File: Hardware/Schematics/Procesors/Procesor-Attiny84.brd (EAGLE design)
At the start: 27.9 x 27.9 mm, 6 parts

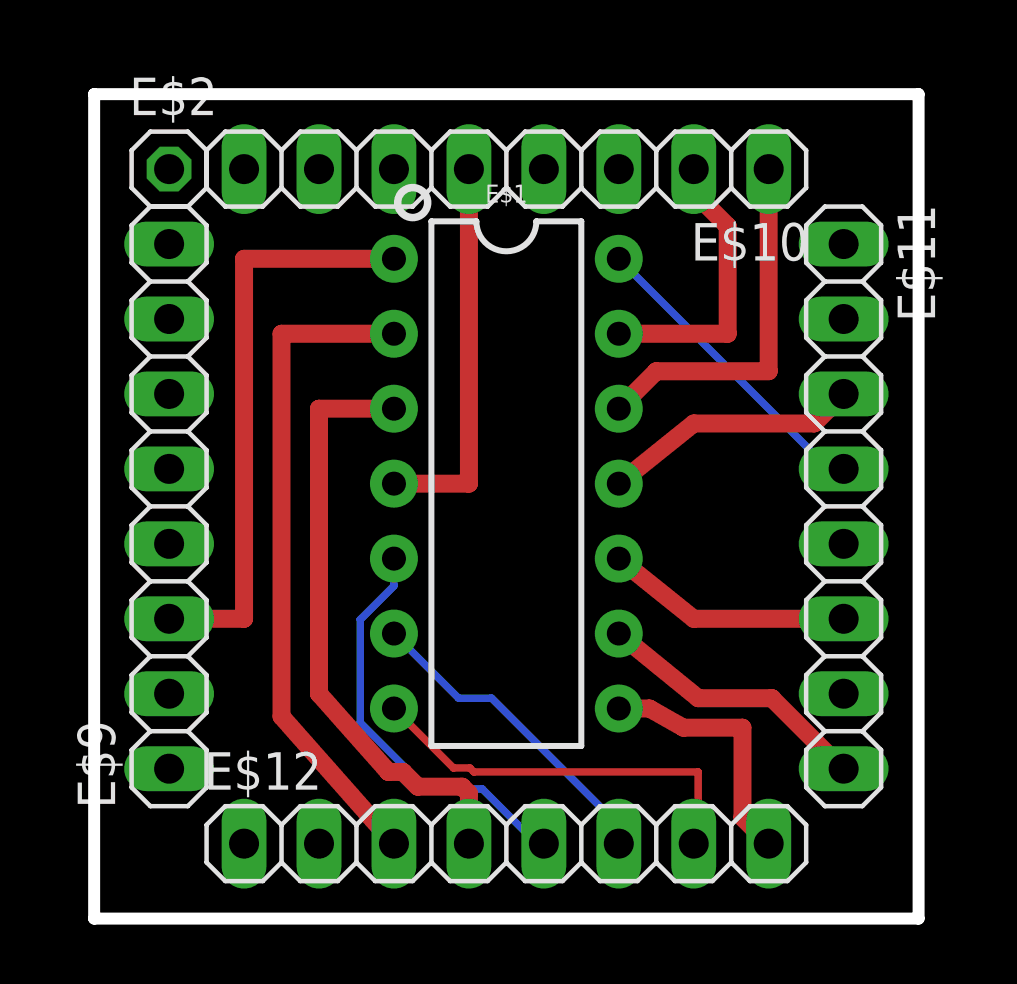
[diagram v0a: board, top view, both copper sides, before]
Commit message: commit
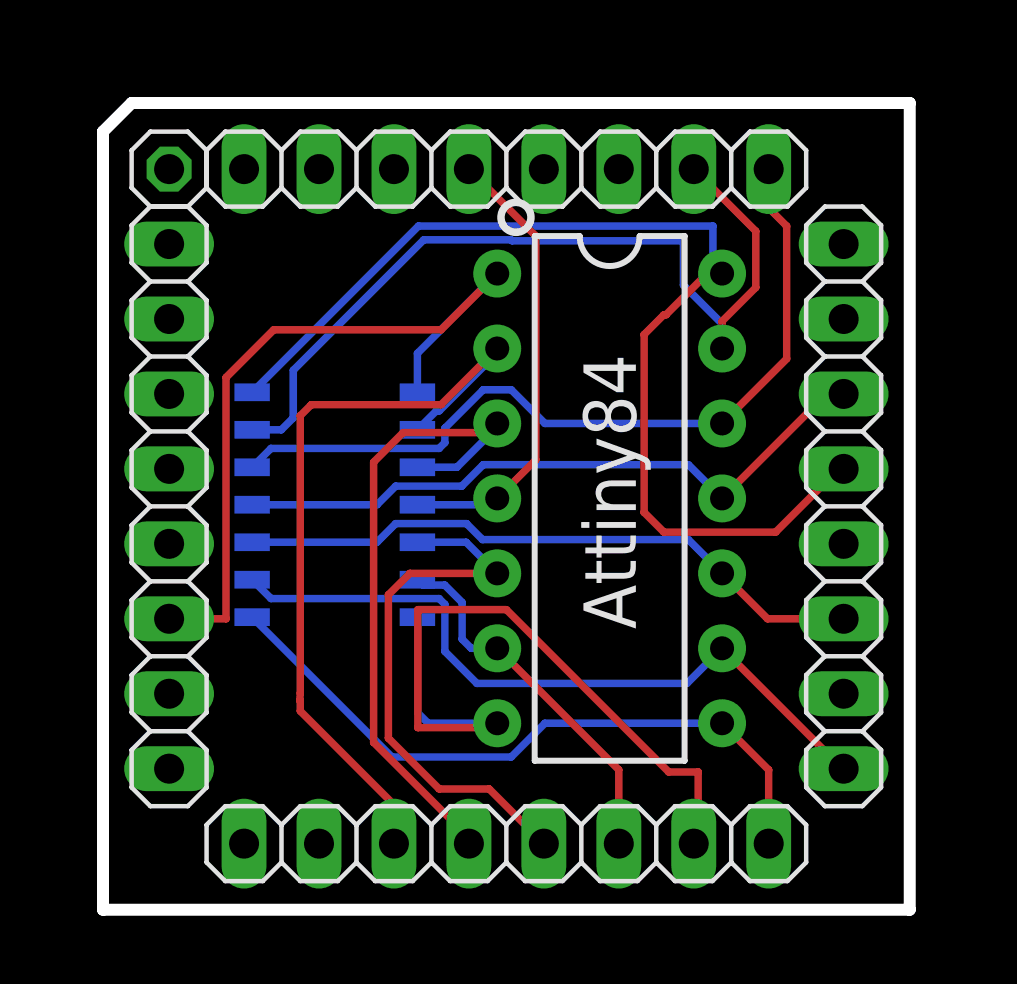
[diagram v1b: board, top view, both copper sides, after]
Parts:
- added E$3: (no value), SparkFun-IC-Microcontroller:SO14
- moved E$1 3.54 mm to (3.50, 0.27)
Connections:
- net S$10: now also E$3.8
- net S$11: now also E$3.10
- net S$12: now also E$3.11
- net S$13: now also E$3.2
- net S$14: now also E$3.3
- net S$15: now also E$3.5
- net S$18: now also E$3.6
- net S$2: now also E$3.4
- net S$3: now also E$3.14
- net S$4: now also E$3.1
- net S$5: now also E$3.9
- net S$6: now also E$3.12
- net S$7: now also E$3.13
- net S$8: now also E$3.7
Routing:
- net S$3: track 10.6 -> 37.1 mm
- net S$7: track 9.75 -> 29.9 mm
- net S$5: track 9.39 -> 24.6 mm
- net S$6: track 12.5 -> 27.6 mm
- net S$10: track 8.66 -> 23.1 mm
- net S$12: track 8.75 -> 22.5 mm
- net S$8: track 13.7 -> 27.1 mm
- net S$11: track 8.34 -> 21.6 mm
- net S$4: track 19.8 -> 25.9 mm
- net S$13: track 22.5 -> 27.4 mm
- net S$15: track 14.0 -> 18.7 mm
- net S$2: track 13.2 -> 15.4 mm
- net S$14: track 20.5 -> 22.4 mm
- net S$18: track 10.9 -> 12.7 mm
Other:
- board size 27.9 x 27.9 mm -> 27.3 x 27.3 mm
- board text added: "Attiny84"
